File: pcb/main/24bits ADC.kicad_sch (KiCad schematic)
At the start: 8 parts

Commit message: fix: symbol libraries in Kicad 6.0
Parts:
- C26, C28: value (none) -> 100n; footprint (none) -> Capacitor_SMD:C_0805_2012Metric_Pad1.15x1.40mm_HandSolder; symbol pHMeter-rescue:C-Device -> Device:C
- C27, C29: value (none) -> 10u; footprint (none) -> Capacitor_SMD:C_0805_2012Metric_Pad1.15x1.40mm_HandSolder; symbol pHMeter-rescue:C-Device -> Device:C
- J8: value (none) -> SJ; footprint (none) -> Jumper:SolderJumper-2_P1.3mm_Open_RoundedPad1.0x1.5mm
- R41: value (none) -> 10k; footprint (none) -> Resistor_SMD:R_0805_2012Metric_Pad1.15x1.40mm_HandSolder; symbol pHMeter-rescue:R-Device -> Device:R
- SJ1: value (none) -> JUMPER-PAD-2-NC_BY_TRACE; footprint (none) -> Jumper:SolderJumper-2_P1.3mm_Open_RoundedPad1.0x1.5mm
- U6: value (none) -> HX711; footprint (none) -> Package_SO:SOIC-16_3.9x9.9mm_P1.27mm
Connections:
- net 3.3V: now also C26.1, C27.1, C28.1, C29.1, R41.1
- net GND: now also C26.2, C27.2
- net LGND: now also C28.2, C29.2
- net at J8.2, U6.15 (RATE): now also R41.2
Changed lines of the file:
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@@
       (effects (font (size 1.4986 1.4986)) (justify right))
     )
-    (property "Value" "" (id 1) (at 82.55 106.68 0)
+    (property "Value" "JUMPER-PAD-2-NC_BY_TRACE" (id 1) (at 82.55 106.68 0)
       (effects (font (size 1.4986 1.4986)) (justify right))
     )
-    (property "Footprint" "" (id 2) (at 90.17 124.46 0)
+    (property "Footprint" "Jumper:SolderJumper-2_P1.3mm_Open_RoundedPad1.0x1.5mm" (id 2) (at 90.17 124.46 0)
       (effects (font (size 1.27 1.27)) hide)
     )
@@
     (pin "2")
   )
-  (symbol (lib_id "pHMeter-rescue:C-Device") (at 96.52 123.825 0) (unit 1)
+  (symbol (lib_id "Device:C") (at 96.52 123.825 0) (unit 1)
     (in_bom yes) (on_board yes)
     (property "Reference" "C26" (id 0) (at 99.695 122.555 0)
       (effects (font (size 1.27 1.27)) (justify left))
     )
-    (property "Value" "" (id 1) (at 97.155 126.365 0)
+    (property "Value" "100n" (id 1) (at 97.155 126.365 0)
       (effects (font (size 1.27 1.27)) (justify left))
     )
-    (property "Footprint" "" (id 2) (at 97.4852 127.635 0)
+    (property "Footprint" "Capacitor_SMD:C_0805_2012Metric_Pad1.15x1.40mm_HandSolder" (id 2) (at 97.4852 127.635 0)
       (effects (font (size 1.27 1.27)) hide)
     )
@@
       (effects (font (size 1.27 1.27)) hide)
     )
+    (pin "1")
+    (pin "2")
   )
-  (symbol (lib_id "pHMeter-rescue:C-Device") (at 104.775 123.825 0) (unit 1)
+  (symbol (lib_id "Device:C") (at 104.775 123.825 0) (unit 1)
     (in_bom yes) (on_board yes)
     (property "Reference" "C27" (id 0) (at 107.95 122.555 0)
       (effects (font (size 1.27 1.27)) (justify left))
     )
-    (property "Value" "" (id 1) (at 105.41 126.365 0)
+    (property "Value" "10u" (id 1) (at 105.41 126.365 0)
       (effects (font (size 1.27 1.27)) (justify left))
     )
-    (property "Footprint" "" (id 2) (at 105.7402 127.635 0)
+    (property "Footprint" "Capacitor_SMD:C_0805_2012Metric_Pad1.15x1.40mm_HandSolder" (id 2) (at 105.7402 127.635 0)
       (effects (font (size 1.27 1.27)) hide)
     )
@@
       (effects (font (size 1.27 1.27)) hide)
     )
+    (pin "1")
+    (pin "2")
   )
-  (symbol (lib_id "pHMeter-rescue:C-Device") (at 122.555 87.63 0) (unit 1)
+  (symbol (lib_id "Device:C") (at 122.555 87.63 0) (unit 1)
     (in_bom yes) (on_board yes)
     (property "Reference" "C28" (id 0) (at 123.825 85.725 0)
       (effects (font (size 1.27 1.27)) (justify left))
     )
-    (property "Value" "" (id 1) (at 123.19 90.17 0)
+    (property "Value" "100n" (id 1) (at 123.19 90.17 0)
       (effects (font (size 1.27 1.27)) (justify left))
     )
-    (property "Footprint" "" (id 2) (at 123.5202 91.44 0)
+    (property "Footprint" "Capacitor_SMD:C_0805_2012Metric_Pad1.15x1.40mm_HandSolder" (id 2) (at 123.5202 91.44 0)
       (effects (font (size 1.27 1.27)) hide)
     )
@@
       (effects (font (size 1.27 1.27)) hide)
     )
+    (pin "1")
+    (pin "2")
   )
-  (symbol (lib_id "pHMeter-rescue:C-Device") (at 130.81 87.63 0) (unit 1)
+  (symbol (lib_id "Device:C") (at 130.81 87.63 0) (unit 1)
     (in_bom yes) (on_board yes)
     (property "Reference" "C29" (id 0) (at 132.08 85.725 0)
       (effects (font (size 1.27 1.27)) (justify left))
     )
-    (property "Value" "" (id 1) (at 131.445 90.17 0)
+    (property "Value" "10u" (id 1) (at 131.445 90.17 0)
       (effects (font (size 1.27 1.27)) (justify left))
     )
-    (property "Footprint" "" (id 2) (at 131.7752 91.44 0)
+    (property "Footprint" "Capacitor_SMD:C_0805_2012Metric_Pad1.15x1.40mm_HandSolder" (id 2) (at 131.7752 91.44 0)
       (effects (font (size 1.27 1.27)) hide)
     )
@@
       (effects (font (size 1.27 1.27)) hide)
     )
+    (pin "1")
+    (pin "2")
   )
   (symbol (lib_id "Bertha_main-eagle-import:SJ") (at 198.755 76.2 180) (unit 1)
@@
       (effects (font (size 1.4986 1.4986)))
     )
-    (property "Value" "" (id 1) (at 198.755 78.74 0)
+    (property "Value" "SJ" (id 1) (at 198.755 78.74 0)
       (effects (font (size 1.4986 1.4986)))
     )
-    (property "Footprint" "" (id 2) (at 198.755 76.2 0)
+    (property "Footprint" "Jumper:SolderJumper-2_P1.3mm_Open_RoundedPad1.0x1.5mm" (id 2) (at 198.755 76.2 0)
       (effects (font (size 1.27 1.27)) hide)
     )
@@
     (pin "2")
   )
-  (symbol (lib_id "pHMeter-rescue:R-Device") (at 192.405 71.12 0) (unit 1)
+  (symbol (lib_id "Device:R") (at 192.405 71.12 0) (unit 1)
     (in_bom yes) (on_board yes)
     (property "Reference" "R41" (id 0) (at 194.945 73.66 90)
       (effects (font (size 1.27 1.27)) (justify left))
     )
-    (property "Value" "" (id 1) (at 192.405 73.025 90)
+    (property "Value" "10k" (id 1) (at 192.405 73.025 90)
       (effects (font (size 1.27 1.27)) (justify left))
     )
-    (property "Footprint" "" (id 2) (at 190.627 71.12 90)
+    (property "Footprint" "Resistor_SMD:R_0805_2012Metric_Pad1.15x1.40mm_HandSolder" (id 2) (at 190.627 71.12 90)
       (effects (font (size 1.27 1.27)) hide)
     )
@@
       (effects (font (size 1.27 1.27)) hide)
     )
+    (pin "1")
+    (pin "2")
   )
   (symbol (lib_id "bioreactor:HX711") (at 170.815 88.9 0) (unit 1)
@@
       (effects (font (size 1.4986 1.4986)))
     )
-    (property "Value" "" (id 1) (at 169.545 66.5226 0)
+    (property "Value" "HX711" (id 1) (at 169.545 66.5226 0)
       (effects (font (size 1.4986 1.4986)))
     )
-    (property "Footprint" "" (id 2) (at 170.815 115.57 0)
+    (property "Footprint" "Package_SO:SOIC-16_3.9x9.9mm_P1.27mm" (id 2) (at 170.815 115.57 0)
       (effects (font (size 1.27 1.27)) hide)
     )

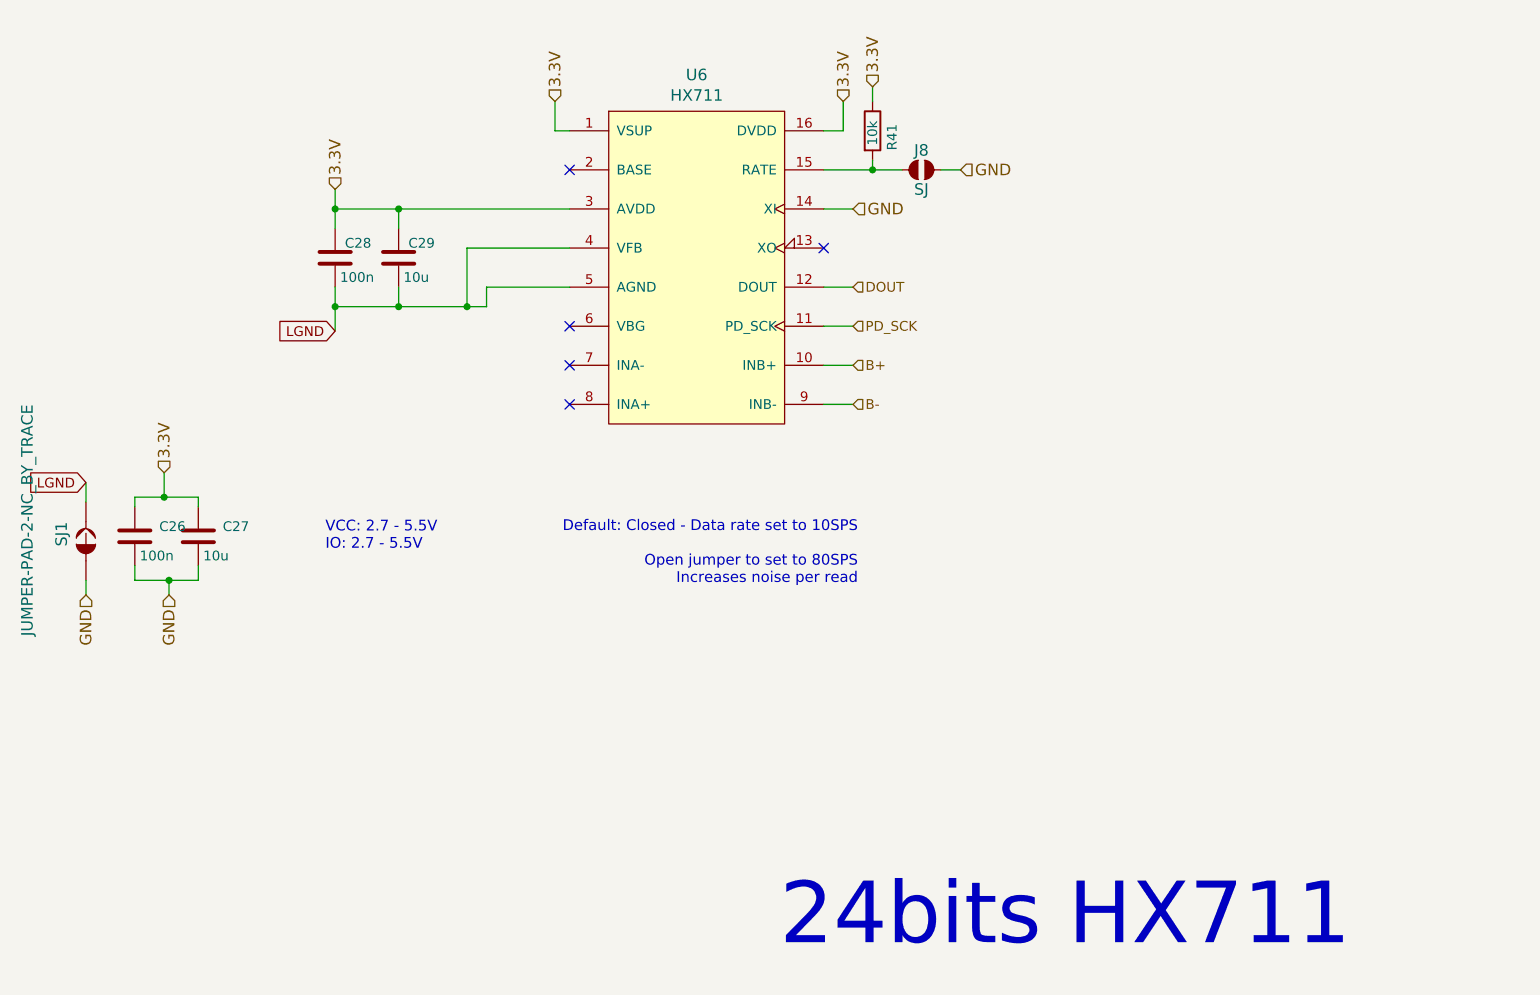
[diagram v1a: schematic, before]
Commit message: fix: standard footprint for R and C, BOM updated
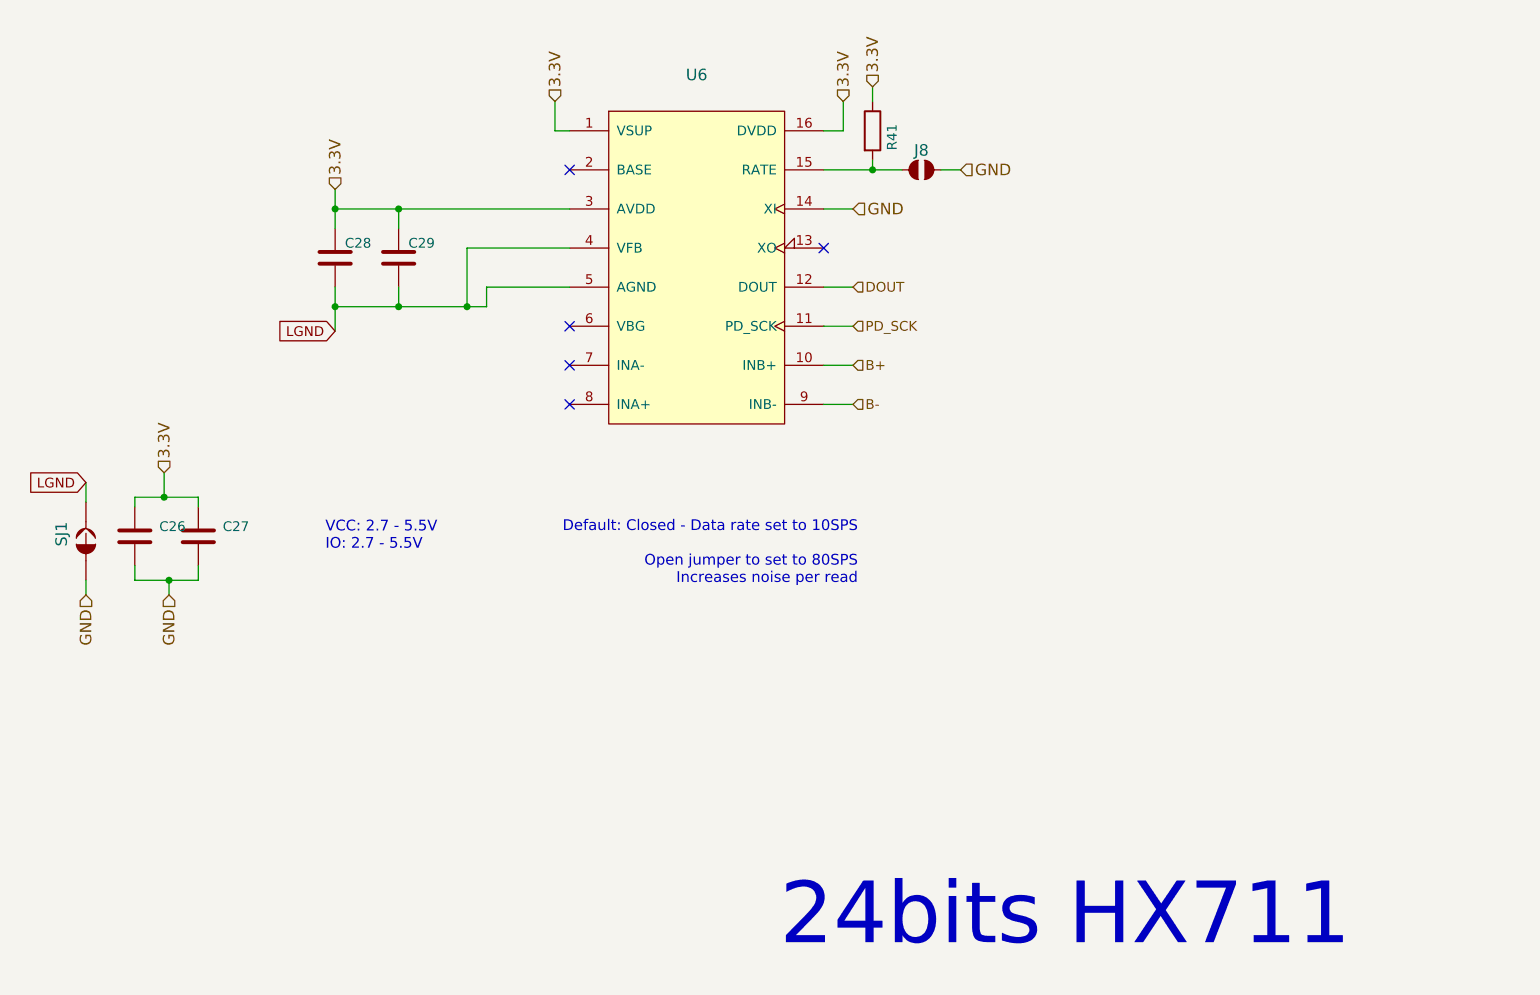
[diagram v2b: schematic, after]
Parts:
- C26, C28: value 100n -> (none); footprint Capacitor_SMD:C_0805_2012Metric_Pad1.15x1.40mm_HandSolder -> (none)
- C27, C29: value 10u -> (none); footprint Capacitor_SMD:C_0805_2012Metric_Pad1.15x1.40mm_HandSolder -> (none); MFN Samsung Electro-Mechanics -> Wurth Elektronik; MFP CL21A106KOQNNNG -> 885012207072; S1PL https://www.mouser.com/ProductDetail/Samsung-Electro-Mechan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 -> https://www.mouser.com/ProductDetail/Wurth-Elektronik/88501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; S1PN 187-CL21A106KOQNNNG -> 710-885012207072
- J8: value SJ -> (none); footprint Jumper:SolderJumper-2_P1.3mm_Open_RoundedPad1.0x1.5mm -> (none)
- R41: value 10k -> (none); footprint Resistor_SMD:R_0805_2012Metric_Pad1.15x1.40mm_HandSolder -> (none)
- SJ1: value JUMPER-PAD-2-NC_BY_TRACE -> (none); footprint Jumper:SolderJumper-2_P1.3mm_Open_RoundedPad1.0x1.5mm -> (none)
- U6: value HX711 -> (none); footprint Package_SO:SOIC-16_3.9x9.9mm_P1.27mm -> (none)
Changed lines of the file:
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@@
       (effects (font (size 1.4986 1.4986)) (justify right))
     )
-    (property "Value" "JUMPER-PAD-2-NC_BY_TRACE" (id 1) (at 82.55 106.68 0)
+    (property "Value" "" (id 1) (at 82.55 106.68 0)
       (effects (font (size 1.4986 1.4986)) (justify right))
     )
-    (property "Footprint" "Jumper:SolderJumper-2_P1.3mm_Open_RoundedPad1.0x1.5mm" (id 2) (at 90.17 124.46 0)
+    (property "Footprint" "" (id 2) (at 90.17 124.46 0)
       (effects (font (size 1.27 1.27)) hide)
     )
@@
       (effects (font (size 1.27 1.27)) (justify left))
     )
-    (property "Value" "100n" (id 1) (at 97.155 126.365 0)
+    (property "Value" "" (id 1) (at 97.155 126.365 0)
       (effects (font (size 1.27 1.27)) (justify left))
     )
-    (property "Footprint" "Capacitor_SMD:C_0805_2012Metric_Pad1.15x1.40mm_HandSolder" (id 2) (at 97.4852 127.635 0)
+    (property "Footprint" "" (id 2) (at 97.4852 127.635 0)
       (effects (font (size 1.27 1.27)) hide)
     )
@@
       (effects (font (size 1.27 1.27)) (justify left))
     )
-    (property "Value" "10u" (id 1) (at 105.41 126.365 0)
+    (property "Value" "" (id 1) (at 105.41 126.365 0)
       (effects (font (size 1.27 1.27)) (justify left))
     )
-    (property "Footprint" "Capacitor_SMD:C_0805_2012Metric_Pad1.15x1.40mm_HandSolder" (id 2) (at 105.7402 127.635 0)
+    (property "Footprint" "" (id 2) (at 105.7402 127.635 0)
       (effects (font (size 1.27 1.27)) hide)
     )
-    (property "Datasheet" "https://www.mouser.com/datasheet/2/585/MLCC-1837944.pdf" (id 3) (at 104.775 123.825 0)
+    (property "Datasheet" "https://www.mouser.com/datasheet/2/445/885012207072-1727745.pdf" (id 3) (at 104.775 123.825 0)
       (effects (font (size 1.27 1.27)) hide)
     )
-    (property "Description" "Multilayer Ceramic Capacitors MLCC - SMD/SMT 16V 10uF X5R 0805 10%" (id 4) (at 104.775 123.825 0)
+    (property "Description" "Multilayer Ceramic Capacitors MLCC - SMD/SMT WCAP-CSGP 0.1uF 0805 10% 25V MLCC " (id 4) (at 104.775 123.825 0)
       (effects (font (size 1.27 1.27)) hide)
     )
-    (property "MFN" "Samsung Electro-Mechanics " (id 5) (at 104.775 123.825 0)
+    (property "MFN" "Wurth Elektronik " (id 5) (at 104.775 123.825 0)
       (effects (font (size 1.27 1.27)) hide)
     )
-    (property "MFP" "CL21A106KOQNNNG " (id 6) (at 104.775 123.825 0)
+    (property "MFP" "885012207072" (id 6) (at 104.775 123.825 0)
       (effects (font (size 1.27 1.27)) hide)
     )
-    (property "S1PL" "https://www.mouser.com/ProductDetail/Samsung-Electro-Mechanics/CL21A106KOQNNNG?qs=hqM3L16%252BxlcMWI7QbqH0LA%3D%3D" (id 7) (at 104.775 123.825 0)
+    (property "S1PL" "https://www.mouser.com/ProductDetail/Wurth-Elektronik/885012207072?qs=0KOYDY2FL28rQMV4504TxA%3D%3D" (id 7) (at 104.775 123.825 0)
       (effects (font (size 1.27 1.27)) hide)
     )
-    (property "S1PN" " 187-CL21A106KOQNNNG " (id 8) (at 104.775 123.825 0)
+    (property "S1PN" "710-885012207072 " (id 8) (at 104.775 123.825 0)
       (effects (font (size 1.27 1.27)) hide)
     )
@@
       (effects (font (size 1.27 1.27)) (justify left))
     )
-    (property "Value" "100n" (id 1) (at 123.19 90.17 0)
+    (property "Value" "" (id 1) (at 123.19 90.17 0)
       (effects (font (size 1.27 1.27)) (justify left))
     )
-    (property "Footprint" "Capacitor_SMD:C_0805_2012Metric_Pad1.15x1.40mm_HandSolder" (id 2) (at 123.5202 91.44 0)
+    (property "Footprint" "" (id 2) (at 123.5202 91.44 0)
       (effects (font (size 1.27 1.27)) hide)
     )
@@
       (effects (font (size 1.27 1.27)) (justify left))
     )
-    (property "Value" "10u" (id 1) (at 131.445 90.17 0)
+    (property "Value" "" (id 1) (at 131.445 90.17 0)
       (effects (font (size 1.27 1.27)) (justify left))
     )
-    (property "Footprint" "Capacitor_SMD:C_0805_2012Metric_Pad1.15x1.40mm_HandSolder" (id 2) (at 131.7752 91.44 0)
+    (property "Footprint" "" (id 2) (at 131.7752 91.44 0)
       (effects (font (size 1.27 1.27)) hide)
     )
-    (property "Datasheet" "https://www.mouser.com/datasheet/2/585/MLCC-1837944.pdf" (id 3) (at 130.81 87.63 0)
+    (property "Datasheet" "https://www.mouser.com/datasheet/2/445/885012207072-1727745.pdf" (id 3) (at 130.81 87.63 0)
       (effects (font (size 1.27 1.27)) hide)
     )
-    (property "Description" "Multilayer Ceramic Capacitors MLCC - SMD/SMT 16V 10uF X5R 0805 10%" (id 4) (at 130.81 87.63 0)
+    (property "Description" "Multilayer Ceramic Capacitors MLCC - SMD/SMT WCAP-CSGP 0.1uF 0805 10% 25V MLCC " (id 4) (at 130.81 87.63 0)
       (effects (font (size 1.27 1.27)) hide)
     )
-    (property "MFN" "Samsung Electro-Mechanics " (id 5) (at 130.81 87.63 0)
+    (property "MFN" "Wurth Elektronik " (id 5) (at 130.81 87.63 0)
       (effects (font (size 1.27 1.27)) hide)
     )
-    (property "MFP" "CL21A106KOQNNNG " (id 6) (at 130.81 87.63 0)
+    (property "MFP" "885012207072" (id 6) (at 130.81 87.63 0)
       (effects (font (size 1.27 1.27)) hide)
     )
-    (property "S1PL" "https://www.mouser.com/ProductDetail/Samsung-Electro-Mechanics/CL21A106KOQNNNG?qs=hqM3L16%252BxlcMWI7QbqH0LA%3D%3D" (id 7) (at 130.81 87.63 0)
+    (property "S1PL" "https://www.mouser.com/ProductDetail/Wurth-Elektronik/885012207072?qs=0KOYDY2FL28rQMV4504TxA%3D%3D" (id 7) (at 130.81 87.63 0)
       (effects (font (size 1.27 1.27)) hide)
     )
-    (property "S1PN" " 187-CL21A106KOQNNNG " (id 8) (at 130.81 87.63 0)
+    (property "S1PN" "710-885012207072 " (id 8) (at 130.81 87.63 0)
       (effects (font (size 1.27 1.27)) hide)
     )
@@
       (effects (font (size 1.4986 1.4986)))
     )
-    (property "Value" "SJ" (id 1) (at 198.755 78.74 0)
+    (property "Value" "" (id 1) (at 198.755 78.74 0)
       (effects (font (size 1.4986 1.4986)))
     )
-    (property "Footprint" "Jumper:SolderJumper-2_P1.3mm_Open_RoundedPad1.0x1.5mm" (id 2) (at 198.755 76.2 0)
+    (property "Footprint" "" (id 2) (at 198.755 76.2 0)
       (effects (font (size 1.27 1.27)) hide)
     )
@@
       (effects (font (size 1.27 1.27)) (justify left))
     )
-    (property "Value" "10k" (id 1) (at 192.405 73.025 90)
+    (property "Value" "" (id 1) (at 192.405 73.025 90)
       (effects (font (size 1.27 1.27)) (justify left))
     )
-    (property "Footprint" "Resistor_SMD:R_0805_2012Metric_Pad1.15x1.40mm_HandSolder" (id 2) (at 190.627 71.12 90)
+    (property "Footprint" "" (id 2) (at 190.627 71.12 90)
       (effects (font (size 1.27 1.27)) hide)
     )
@@
       (effects (font (size 1.4986 1.4986)))
     )
-    (property "Value" "HX711" (id 1) (at 169.545 66.5226 0)
+    (property "Value" "" (id 1) (at 169.545 66.5226 0)
       (effects (font (size 1.4986 1.4986)))
     )
-    (property "Footprint" "Package_SO:SOIC-16_3.9x9.9mm_P1.27mm" (id 2) (at 170.815 115.57 0)
+    (property "Footprint" "" (id 2) (at 170.815 115.57 0)
       (effects (font (size 1.27 1.27)) hide)
     )
